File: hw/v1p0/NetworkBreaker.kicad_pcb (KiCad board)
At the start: 2 copper layers, 20.6 x 91.4 mm, 27 parts, among them J1 8P8C_Shielded, J2 8P8C_Shielded, J4 USB_B_Micro, J5 Conn_01x06, K1 M4-5HAW, K2 M4-5HAW, K3 M4-5HAW, K4 M4-5HAW, U1 ULN2003, U2 FT230XS

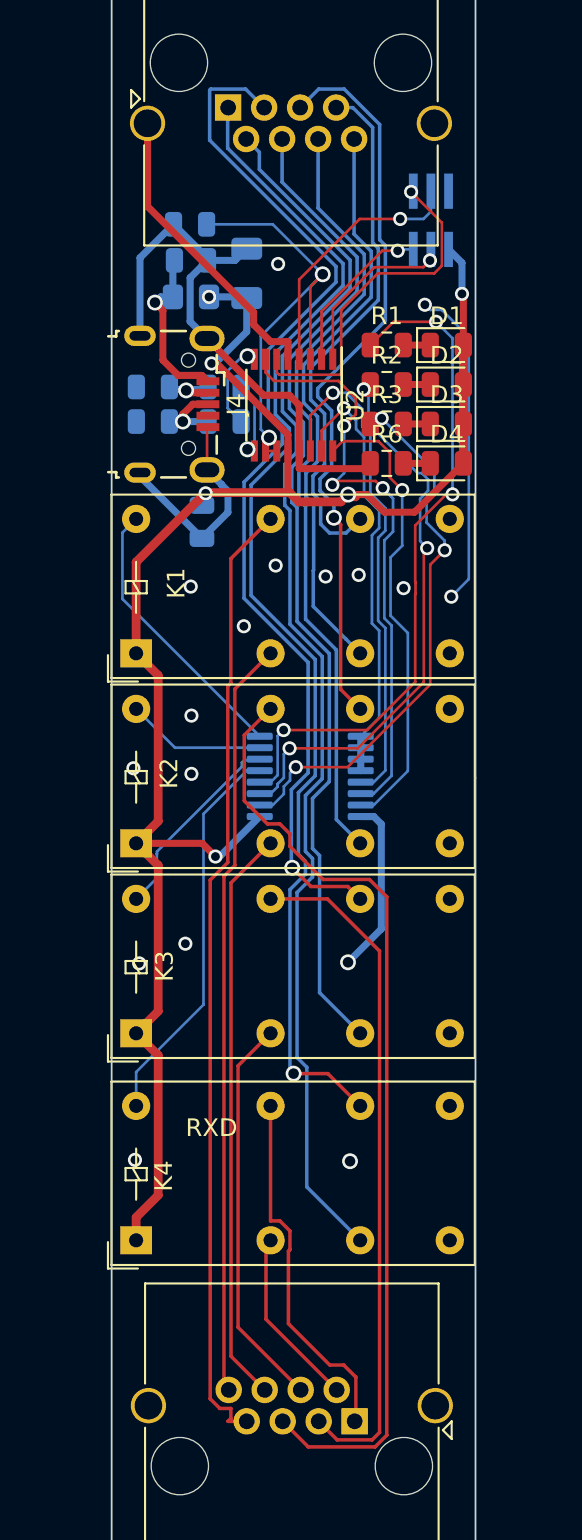
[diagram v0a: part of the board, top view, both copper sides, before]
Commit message: Updated
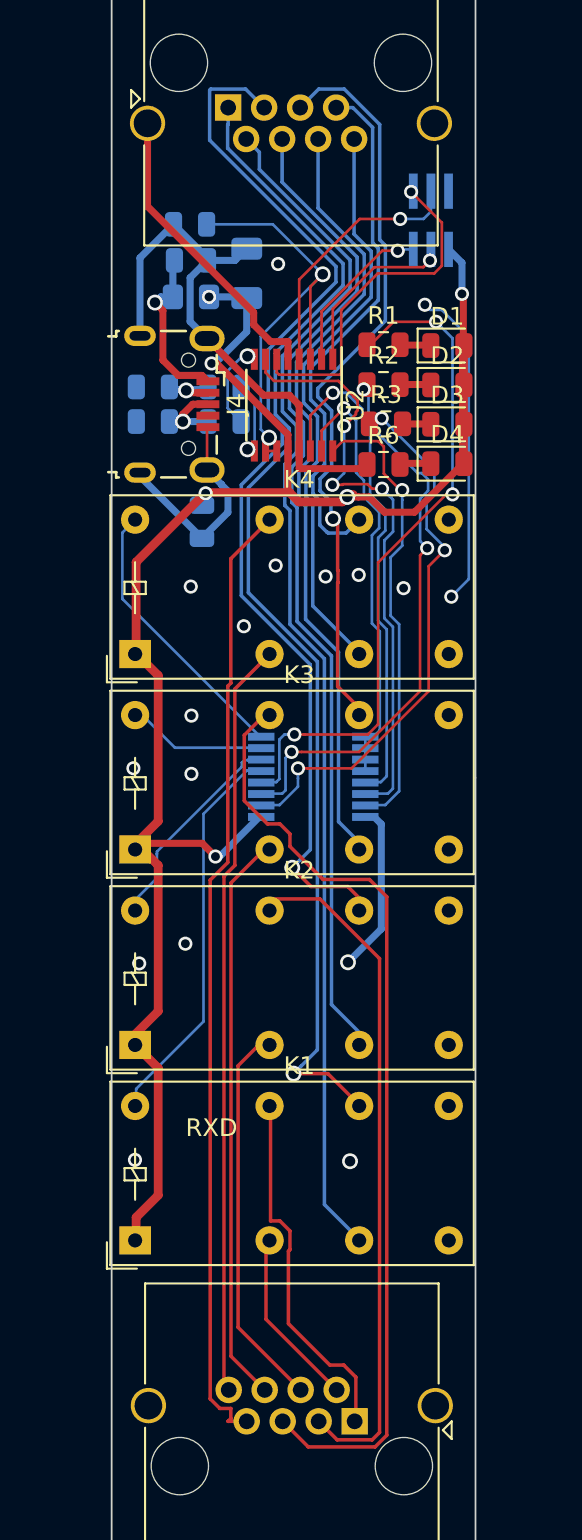
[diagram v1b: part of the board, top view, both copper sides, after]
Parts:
- moved K1 33.3 mm to (201.3, 126.2)
- moved K4 33.2 mm to (201.3, 92.9)
- moved K2 11.4 mm to (201.3, 115.1)
- moved K3 10.4 mm to (201.3, 104.0)
- moved R6 0.20 mm to (215.4, 82.2)
- moved R1 0.19 mm to (215.4, 75.4)
- moved R2 0.19 mm to (215.4, 77.7)
- moved U1 0.17 mm to (211.4, 99.9)
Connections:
- net /LED_1_CTRL renamed LED_1_CTRL
- net /LED_2_CTRL renamed LED_2_CTRL
- net /LED_3_CTRL renamed LED_3_CTRL
- J1 pad 1: /ENET1_PIN1 -> ENET1_PIN1
- J1 pad 2: /ENET1_PIN2 -> ENET1_PIN2
- J1 pad 3: /ENET1_PIN3 -> ENET1_PIN3
- J1 pad 4: /ENET1_PIN4 -> ENET1_PIN4
- J1 pad 5: /ENET1_PIN5 -> ENET1_PIN5
- J1 pad 6: /ENET1_PIN6 -> ENET1_PIN6
- J1 pad 7: /ENET1_PIN7 -> ENET1_PIN7
- J1 pad 8: /ENET1_PIN8 -> ENET1_PIN8
- J2 pad 1: /ENET2_PIN1 -> ENET2_PIN1
- J2 pad 2: /ENET2_PIN2 -> ENET2_PIN2
- J2 pad 3: /ENET2_PIN3 -> ENET2_PIN3
- J2 pad 4: /ENET2_PIN4 -> ENET2_PIN4
- J2 pad 5: /ENET2_PIN5 -> ENET2_PIN5
- J2 pad 6: /ENET2_PIN6 -> ENET2_PIN6
- J2 pad 7: /ENET2_PIN7 -> ENET2_PIN7
- J2 pad 8: /ENET2_PIN8 -> ENET2_PIN8
- J4 pad 4: (no net) -> Net-(J4-Pad4)
- K1 pad 11: /ENET1_PIN8 -> ENET1_PIN2
- K1 pad 12: /ENET2_PIN8 -> ENET2_PIN2
- K1 pad 14: (no net) -> ENET3_PIN2
- K1 pad 21: /ENET1_PIN7 -> ENET1_PIN1
- K1 pad 22: /ENET2_PIN7 -> ENET2_PIN1
- K1 pad 24: (no net) -> ENET3_PIN1
- K1 pad A2: /RELAY_1_CTRL -> RELAY_4_CTRL
- K2 pad 11: /ENET1_PIN6 -> ENET1_PIN4
- K2 pad 12: /ENET2_PIN6 -> ENET2_PIN4
- K2 pad 14: (no net) -> ENET3_PIN4
- K2 pad 21: /ENET1_PIN5 -> ENET1_PIN3
- K2 pad 22: /ENET2_PIN5 -> ENET2_PIN3
- K2 pad 24: (no net) -> ENET3_PIN3
- K2 pad A2: /RELAY_2_CTRL -> RELAY_3_CTRL
- K3 pad 11: /ENET1_PIN4 -> ENET1_PIN6
- K3 pad 12: /ENET2_PIN4 -> ENET2_PIN6
- K3 pad 14: (no net) -> ENET3_PIN6
- K3 pad 21: /ENET1_PIN3 -> ENET1_PIN5
- K3 pad 22: /ENET2_PIN3 -> ENET2_PIN5
- K3 pad 24: (no net) -> ENET3_PIN5
- K3 pad A2: /RELAY_3_CTRL -> RELAY_2_CTRL
- K4 pad 11: /ENET1_PIN2 -> ENET1_PIN8
- K4 pad 12: /ENET2_PIN2 -> ENET2_PIN8
- K4 pad 14: (no net) -> ENET3_PIN8
- K4 pad 21: /ENET1_PIN1 -> ENET1_PIN7
- K4 pad 22: /ENET2_PIN1 -> ENET2_PIN7
- K4 pad 24: (no net) -> ENET3_PIN7
- K4 pad A2: /RELAY_4_CTRL -> RELAY_1_CTRL
- U1 pad 13: /RELAY_4_CTRL -> RELAY_4_CTRL
- U1 pad 14: /RELAY_3_CTRL -> RELAY_3_CTRL
- U1 pad 15: /RELAY_2_CTRL -> RELAY_2_CTRL
- U1 pad 16: /RELAY_1_CTRL -> RELAY_1_CTRL
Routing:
- net /ENET2_PIN2: track 70.3 -> 0.00 mm
- net ENET2_PIN2: track 0.00 -> 68.8 mm
- net /ENET2_PIN1: track 67.3 -> 0.00 mm, vias 1 -> 0
- net ENET2_PIN1: track 0.00 -> 67.1 mm, vias 0 -> 1
- net ENET2_PIN3: track 0.00 -> 60.1 mm, vias 0 -> 1
- net /ENET2_PIN3: track 59.9 -> 0.00 mm, vias 1 -> 0
- net /ENET2_PIN4: track 57.0 -> 0.00 mm
- net ENET2_PIN4: track 0.00 -> 56.3 mm
- net ENET1_PIN7: track 0.00 -> 54.6 mm
- net /ENET1_PIN7: track 54.6 -> 0.00 mm
- net ENET1_PIN5: track 0.00 -> 53.9 mm
- net /ENET1_PIN5: track 53.9 -> 0.00 mm
- net ENET2_PIN6: track 0.00 -> 44.6 mm
- net /ENET2_PIN6: track 44.6 -> 0.00 mm
- net ENET1_PIN8: track 0.00 -> 43.0 mm
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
